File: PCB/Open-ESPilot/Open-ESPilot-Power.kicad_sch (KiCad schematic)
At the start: 16 parts, among them J15 VOUT, J2 VIN, J3 GND, M1 Clone "MP1584" module, U2 AMS1117-3.3, U3 INA219AxD

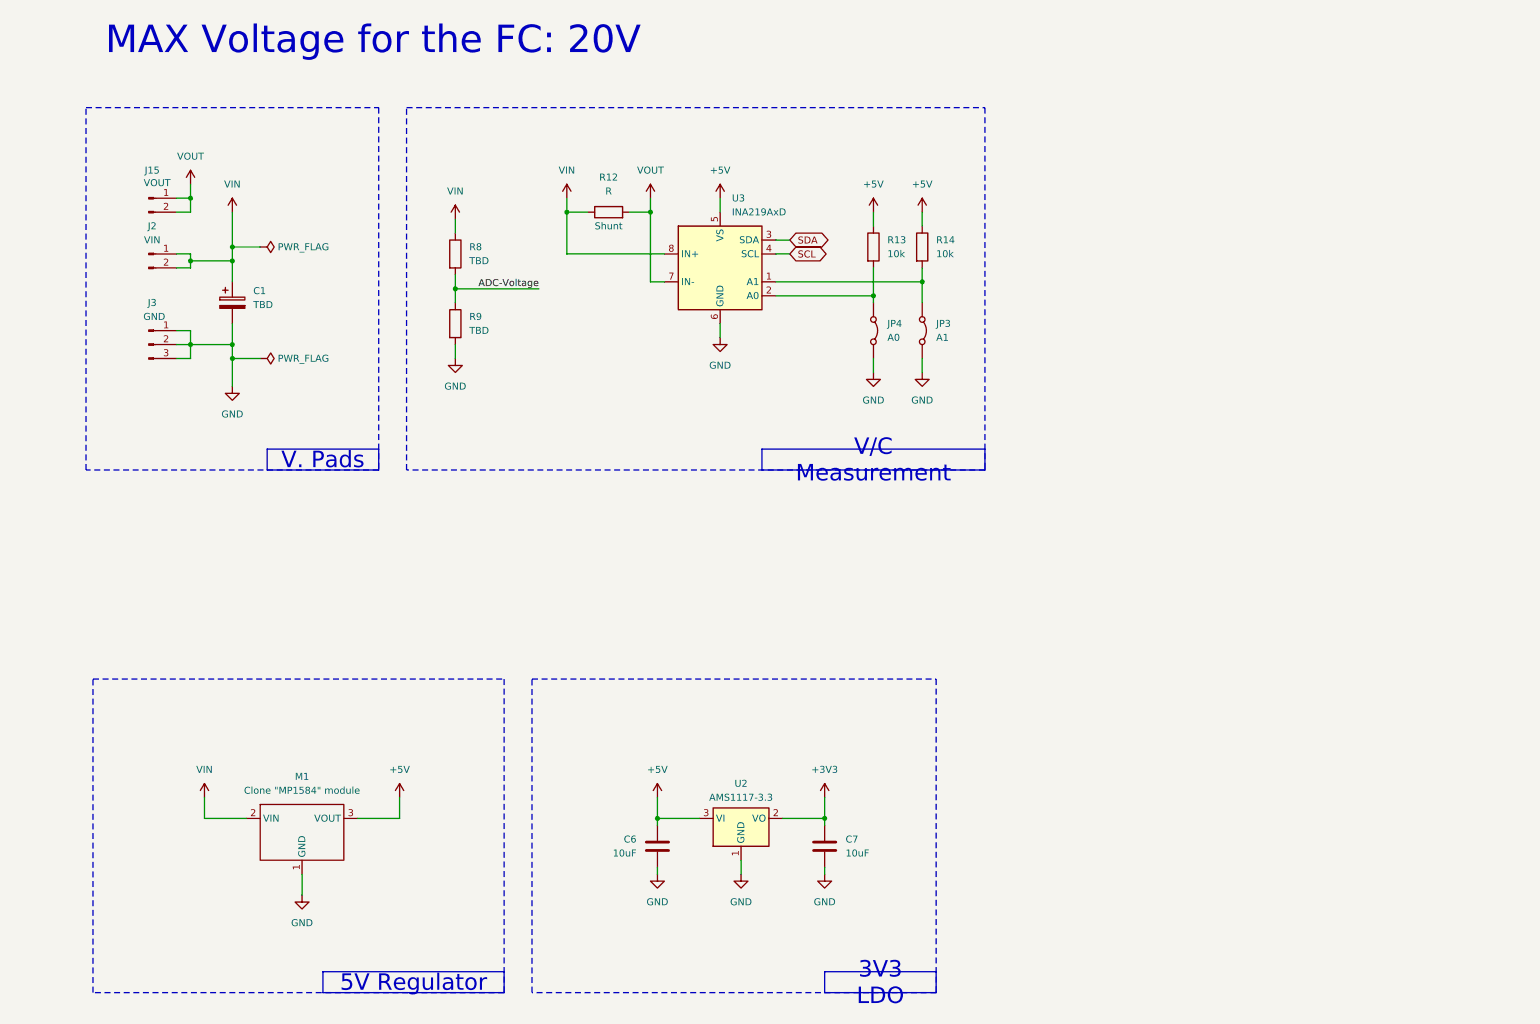
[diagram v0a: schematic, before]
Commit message: Schematic Fixes
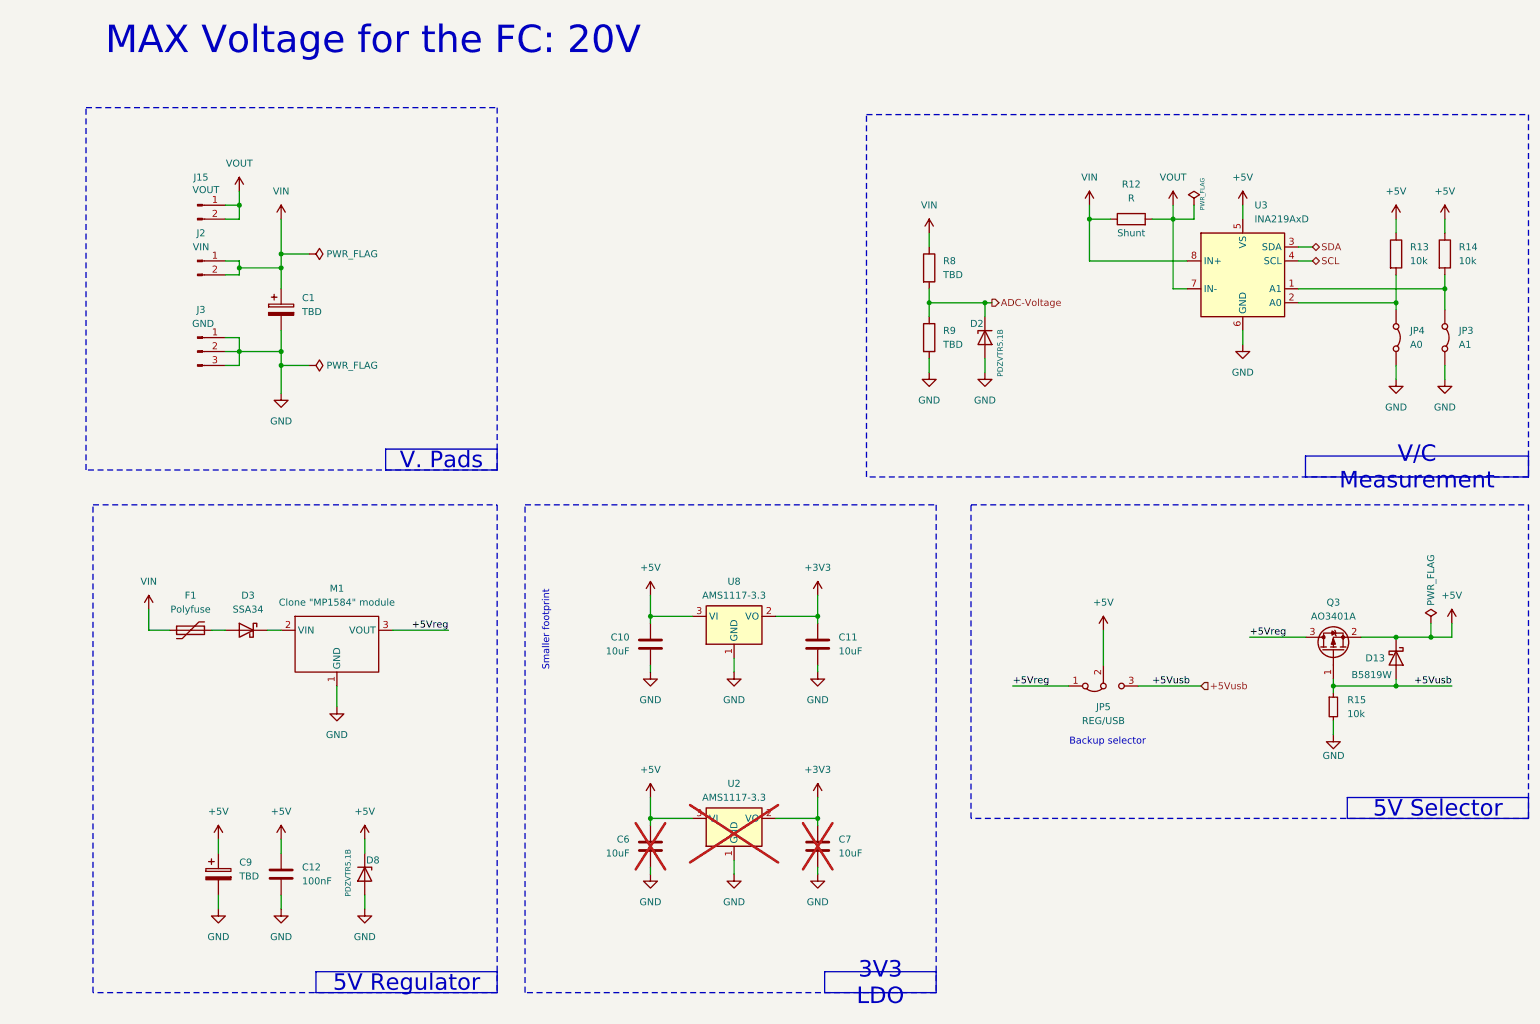
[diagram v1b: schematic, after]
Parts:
- added C10, C11: 10uF, symbol Device:C
- added C12: 100nF, symbol Device:C
- added C9: TBD, symbol Device:C_Polarized
- added D13: B5819W, Diode_SMD:D_SOD-123, symbol Device:D_Schottky
- added D2, D8: PDZVTR5.1B, Diode_SMD:D_SOD-128, symbol Device:D_Zener
- added D3: SSA34, Diode_SMD:D_SMA, symbol Device:D_Schottky
- added F1: Polyfuse, symbol Device:Polyfuse
- added JP5: REG/USB, symbol Jumper:Jumper_3_Bridged12
- added Q3: AO3401A, Package_TO_SOT_SMD:SOT-23, symbol Transistor_FET:AO3401A
- added R15: 10k, Resistor_SMD:R_0603_1608Metric_Pad0.98x0.95mm_HandSolder, symbol Device:R_Small
- added U8: AMS1117-3.3, Package_TO_SOT_SMD:SOT-89-3, symbol Regulator_Linear:AMS1117-3.3
- C6, C7, U2: now not fitted; now left out of the parts list
- M1: footprint Clone "MP1584" module:Clone _MP1584_ module -> Clone _MP1584_ module:Clone _MP1584_ module; symbol Clone {dblquote}MP1584{dblquote} module:Clone_{dblquote}MP1584{dblquote}_module -> Clone _MP1584_ module:Clone _MP1584_ module
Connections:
- net +3V3: now also C11.1, U8.2 (VO)
- net +5V: now also C10.1, C12.1, C9.1, D13.1 (K), D8.1 (K), JP5.2 (C), Q3.2 (S), U8.3 (VI); no longer M1.3 (VOUT)
- net ADC-Voltage: now also D2.1 (K)
- net GND: now also C10.2, C11.2, C12.2, C9.2, D2.2 (A), D8.2 (A), R15.2, U8.1 (GND)
- net VIN: now also F1.1; no longer M1.2 (VIN)
- new net: D3.1 (K), M1.2 (VIN)
- new net: D3.2 (A), F1.2
- new net +5Vreg: JP5.1 (A), M1.3 (VOUT), Q3.3 (D)
- new net +5Vusb: D13.2 (A), JP5.3 (B), Q3.1 (G), R15.1
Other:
- note added: "Backup selector"
- note added: "Smaller footprint"
- moved on the sheet: C1, J15, J2, J3, JP3, JP4, M1, R12, R13, R14, R8, R9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
